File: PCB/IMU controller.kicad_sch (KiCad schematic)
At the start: 38 parts, among them J1 Conn_01x05, U1 NRF52810-QFAA-R, U2 FC31M2-32.768-N09LLDT, U3 BMI270, U6 PTS526SMG15SMTR21 LFS, X1 S3232000081040

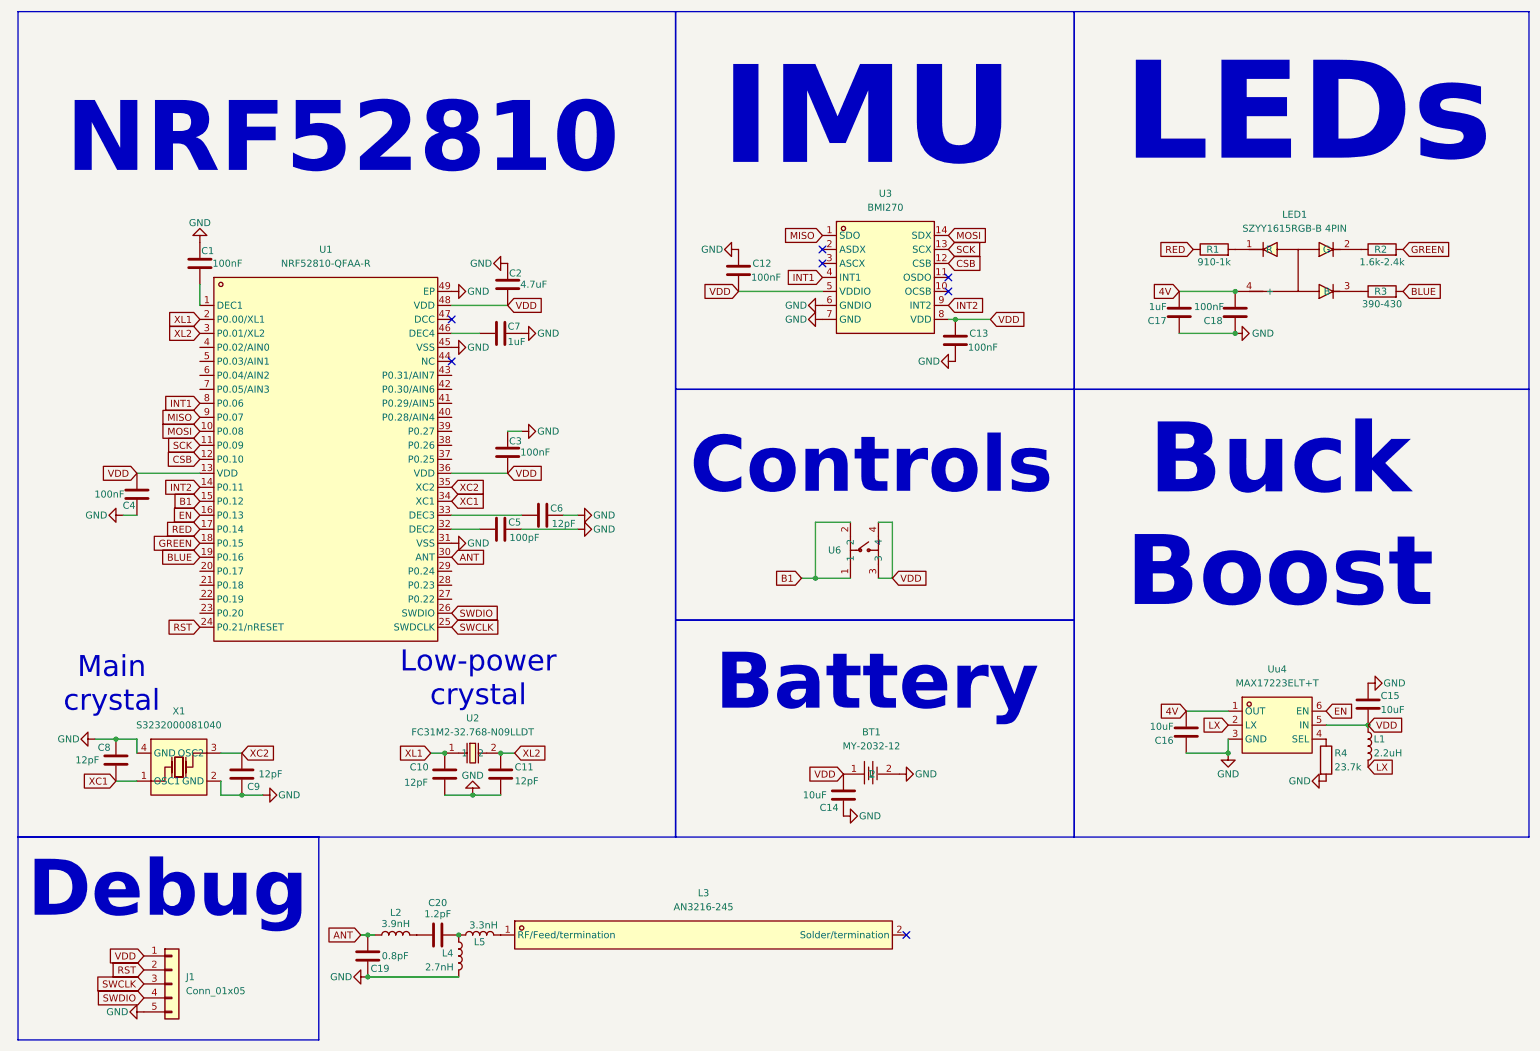
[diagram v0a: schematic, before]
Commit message: added updated PCB files
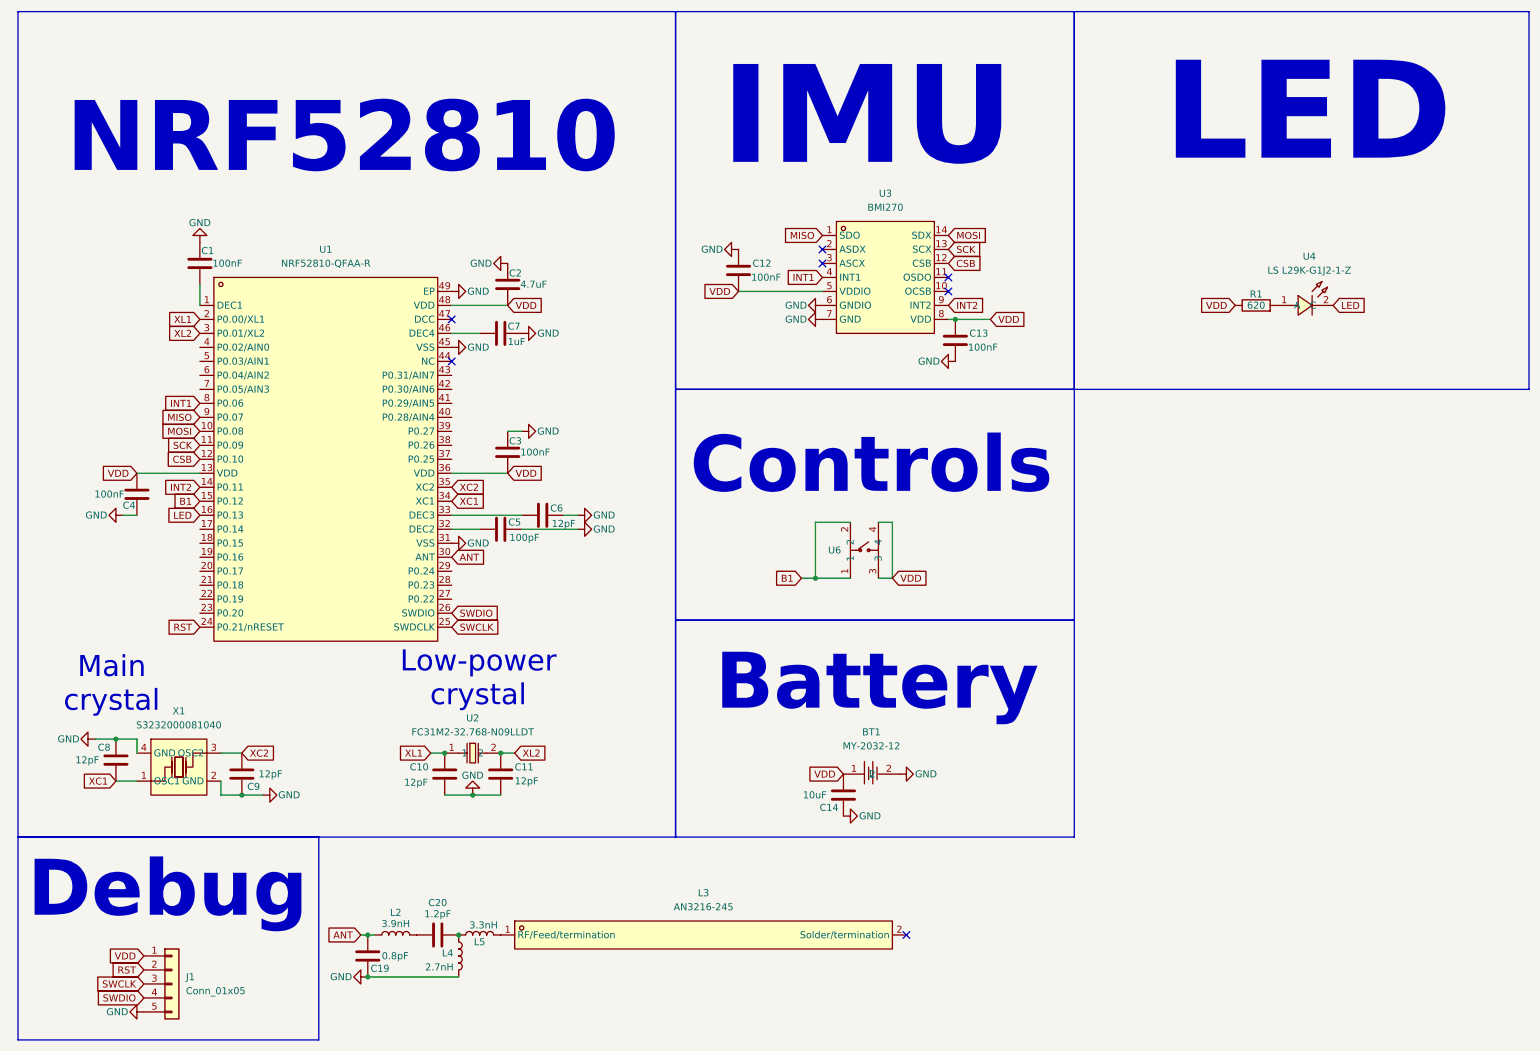
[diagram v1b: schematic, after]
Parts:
- removed C15, C16: 10uF, Capacitor_SMD:C_0805_2012Metric, symbol Device:C
- removed C17: 1uF, Capacitor_SMD:C_0603_1608Metric, symbol Device:C
- removed C18: 100nF, Capacitor_SMD:C_0402_1005Metric, symbol Device:C
- removed L1: 2.2uH, Inductor_SMD:L_0805_2012Metric, symbol Device:L
- removed LED1: SZYY1615RGB-B 4PIN, EasyEDA:LED-SMD_4P-L1.6-W1.5-TR-1, symbol EasyEDA:SZYY1615RGB-B4PIN
- removed R2: 1.6k-2.4k, Resistor_SMD:R_0603_1608Metric, symbol Device:R
- removed R3: 390-430, Resistor_SMD:R_0603_1608Metric, symbol Device:R
- removed R4: 23.7k, Resistor_SMD:R_0603_1608Metric, symbol Device:R
- removed Uu4: MAX17223ELT+T, EasyEDA:UDFN-6_L2.0-W2.0-P0.65-BL, symbol EasyEDA:MAX17223ELT+T
- added U4: LS L29K-G1J2-1-Z, EasyEDA:LED-SMD_L1.3-W0.8-LS1.7-FD, symbol EasyEDA:LSL29K-G1J2-1-Z
- R1: value 910-1k -> 620
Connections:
- net VDD: now also R1.1
- net at R1.2: now also U4.1 (A)
- net BLUE: no longer names the net of U1.19 (P0.16)
- net EN renamed LED
- net LED: now also U4.2 (C)
- net GREEN: no longer names the net of U1.18 (P0.15)
- net RED: no longer names the net of U1.17 (P0.14)
- net RED: no longer R1.1
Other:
- note added: "LED"
- note removed: "Buck Boost"
- note removed: "LEDs"
